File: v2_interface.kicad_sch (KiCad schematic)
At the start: 40 parts, among them J301 DMR-09PGG, J302 PH-2x3SG, Q301 2N7002K, Q302 2N7002K, Q303 2N7002K, Q304 2N7002K, U301 SLG46826G, U302 PCA9515AD, U303 MCP4725A0T-ECH, U304 MCP3424x-xSL, U305 MCP9701A-E_TO

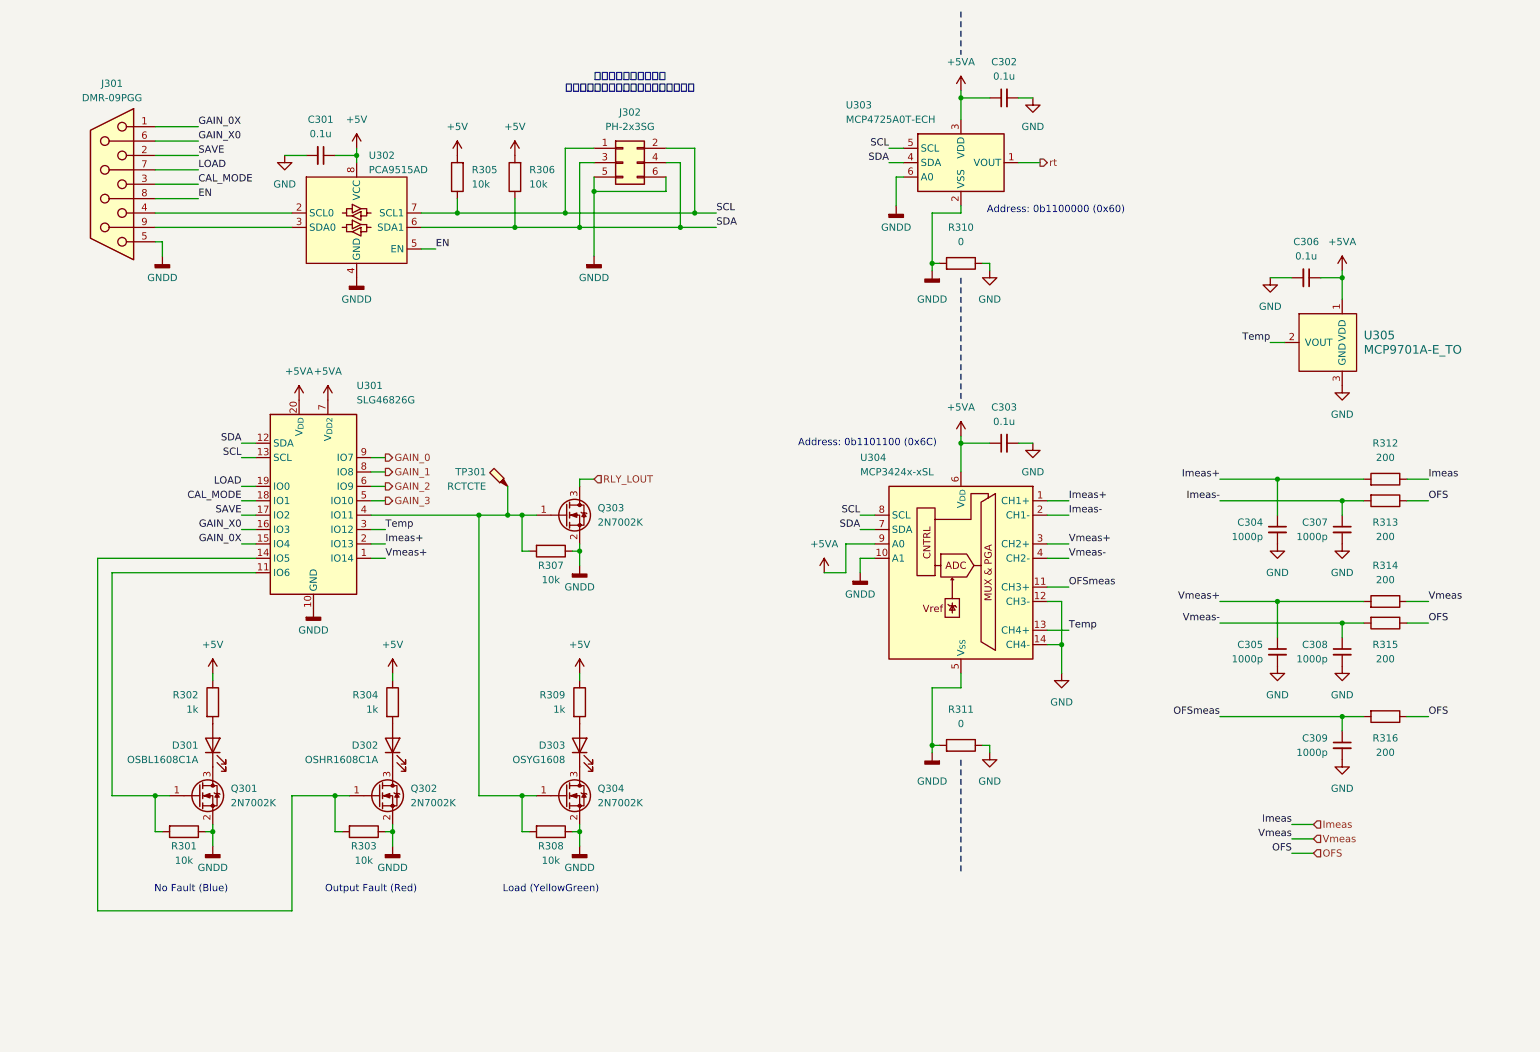
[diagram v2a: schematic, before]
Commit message: kannsei
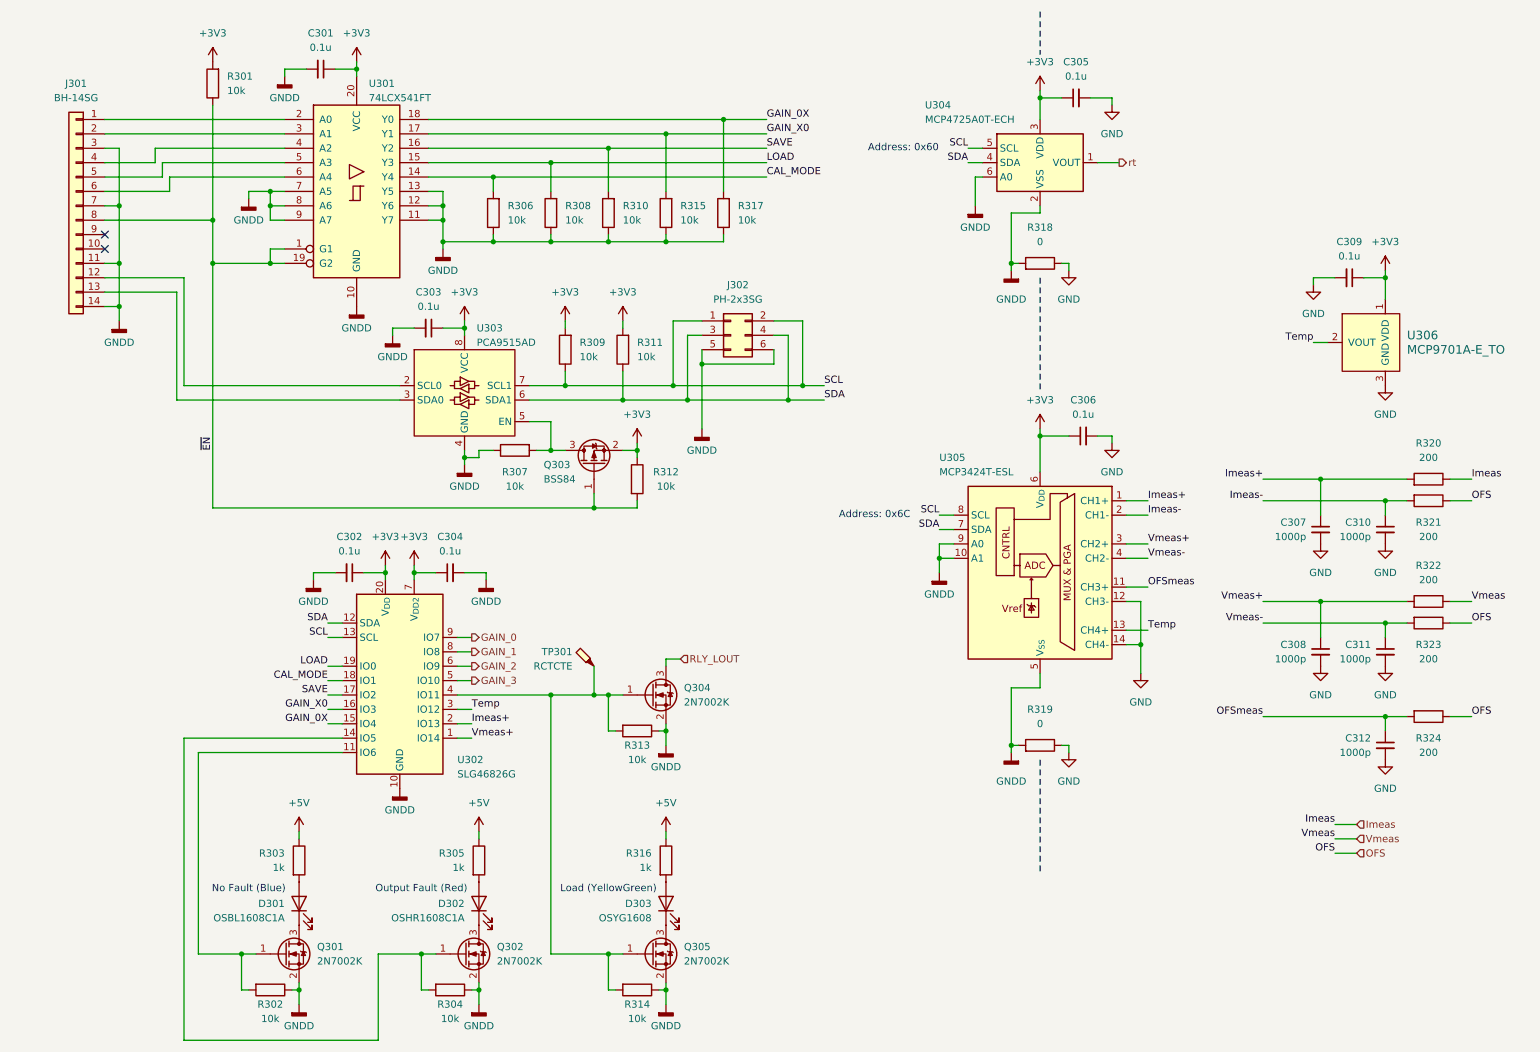
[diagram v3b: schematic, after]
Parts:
- removed J301: DMR-09PGG, symbol Connector:DE9_Socket
- removed R305: 10k, Resistor_SMD:R_0603_1608Metric, symbol Device:R
- removed U302: PCA9515AD, Package_SO:SOIC-8_3.9x4.9mm_P1.27mm, symbol AM_PLD:PCA9515AD
- added C302, C303, C304: 0.1u, Capacitor_SMD:C_0603_1608Metric, symbol Device:C_Small
- added J301: BH-14SG, Connector_IDC:IDC-Header_2x07_P2.54mm_Vertical, symbol Connector_Generic:Conn_01x14
- added Q303: BSS84, Package_TO_SOT_SMD:SOT-23, symbol Transistor_FET:BSS84
- added R301, R307, R308, R309, R310, R311, R312, R315, R317: 10k, Resistor_SMD:R_0603_1608Metric, symbol Device:R
- added U301: 74LCX541FT, Package_SO:TSSOP-20_4.4x6.5mm_P0.65mm, symbol 74xx:74LS541
- added U303: PCA9515AD, Package_SO:SOIC-8_3.9x4.9mm_P1.27mm, symbol AM_PLD:PCA9515AD
- TP301: footprint (none) -> AM_Conn_TP:RCTCE
- U305: renamed from U304; value MCP3424x-xSL -> MCP3424T-ESL
- renumbered C302 to C305, C303 to C306, C304 to C307, C305 to C308, C306 to C309, C307 to C310, C308 to C311, C309 to C312, Q303 to Q304, Q304 to Q305, R301 to R302, R302 to R303, R303 to R304, R304 to R305, R307 to R313, R308 to R314, R309 to R316, R310 to R318, R311 to R319, R312 to R320, R313 to R321, R314 to R322, R315 to R323, R316 to R324, U301 to U302, U303 to U304, U305 to U306
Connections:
- net +5V: no longer C301.1, R306.2
- net CAL_MODE: now also R306.2, U301.14 (Y4)
- net GAIN_0X: now also R317.2, U301.18 (Y0)
- net GAIN_X0: now also R315.2, U301.17 (Y1)
- net GND: no longer C301.2
- net GNDD: now also C301.2, R306.1, U305.9 (A0), C302.2, C303.2, C304.2, J301.11 (Pin_11), J301.14 (Pin_14), J301.3 (Pin_3), J301.7 (Pin_7), R307.1, R308.1, R310.1, R315.1, R317.1, U301.10 (GND), U301.11 (Y7), U301.12 (Y6), U301.13 (Y5), U301.7 (A5), U301.8 (A6), U301.9 (A7), U303.4 (GND)
- net LOAD: now also R308.2, U301.15 (Y3)
- net SAVE: now also R310.2, U301.16 (Y2)
- net SCL: now also R309.1, U303.7 (SCL1)
- net SDA: now also R311.1, U303.6 (SDA1); no longer R306.1
- net +5VA renamed +3V3
- net +3V3: now also C301.1, C302.1, C303.1, C304.1, Q303.2 (S), R301.2, R309.2, R311.2, R312.1, U301.20 (VCC), U303.8 (VCC); no longer U305.9 (A0)
- new net: J301.1 (Pin_1), U301.2 (A0)
- new net: J301.2 (Pin_2), U301.3 (A1)
- new net: J301.4 (Pin_4), U301.4 (A2)
- new net: J301.5 (Pin_5), U301.5 (A3)
- new net: J301.6 (Pin_6), U301.6 (A4)
- new net: J301.12 (Pin_12), U303.2 (SCL0)
- new net: J301.13 (Pin_13), U303.3 (SDA0)
- new net: Q303.3 (D), R307.2, U303.5 (EN)
- new net ~{EN}: J301.8 (Pin_8), Q303.1 (G), R301.1, R312.2, U301.1 (G1), U301.19 (G2)
- no-connect marks 0 -> 2
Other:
- note added: "Address: 0x60"
- note added: "Address: 0x6C"
- note removed: "Address: 0b1100000 (0x60)"
- note removed: "Address: 0b1101100 (0x6C)"
- note removed: "外付け用兼ロジアナ用 使わないときはジャンパーをつけておく"
- company: (none) -> EosinY
- title: (none) -> Analog Controller
- moved on the sheet: C305, C306, C307, C308, C309, C310, C311, C312, D301, D302, D303, Q301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
